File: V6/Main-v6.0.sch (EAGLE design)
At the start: 102 parts, among them J11 AVR_SPI_PROG_3X2NS, M01 JUMPER-SMT_2_NC_PASTE_SILK, M02 JUMPER-SMT_2_NC_PASTE_SILK, M11 JUMPER-SMT_2_NC_PASTE_SILK, M12 JUMPER-SMT_2_NC_PASTE_SILK, Q1 MOSFET-NCHANNEL2N7002PW, Q2 MOSFET-NCHANNEL2N7002PW, U1 ULN2803ADWG4, U10 FSMSMTR, U2 ULN2803ADWG4, U3 UA7805CKTTR, U4 DRV8834RGERTSSOP, U5 DRV8834RGERTSSOP, U7 ATMEGA328P_TQFP, U8 SSA12, U9 FSMSMTR, X1 FH12-16S-1SH, Y1 16MHZ

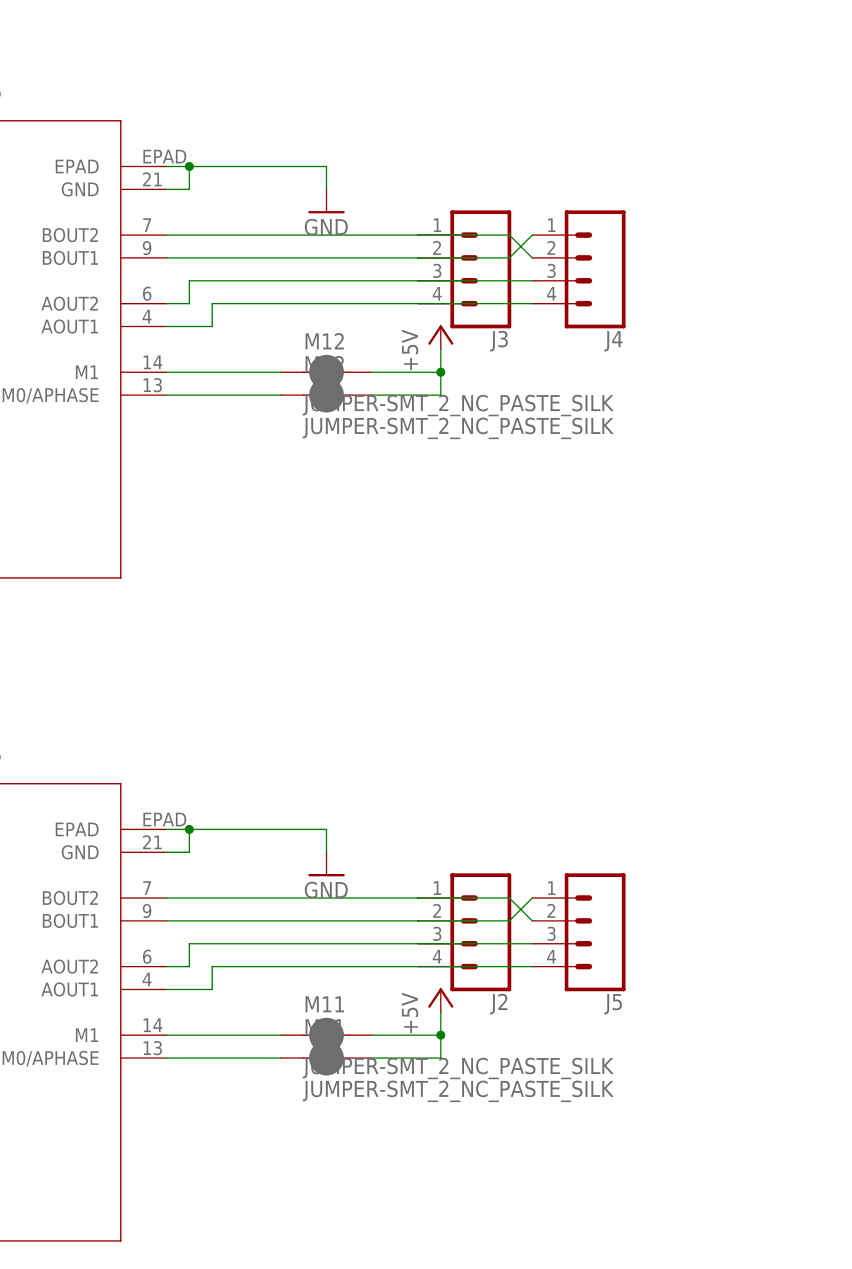
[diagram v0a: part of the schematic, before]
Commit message: V6.0 Updated
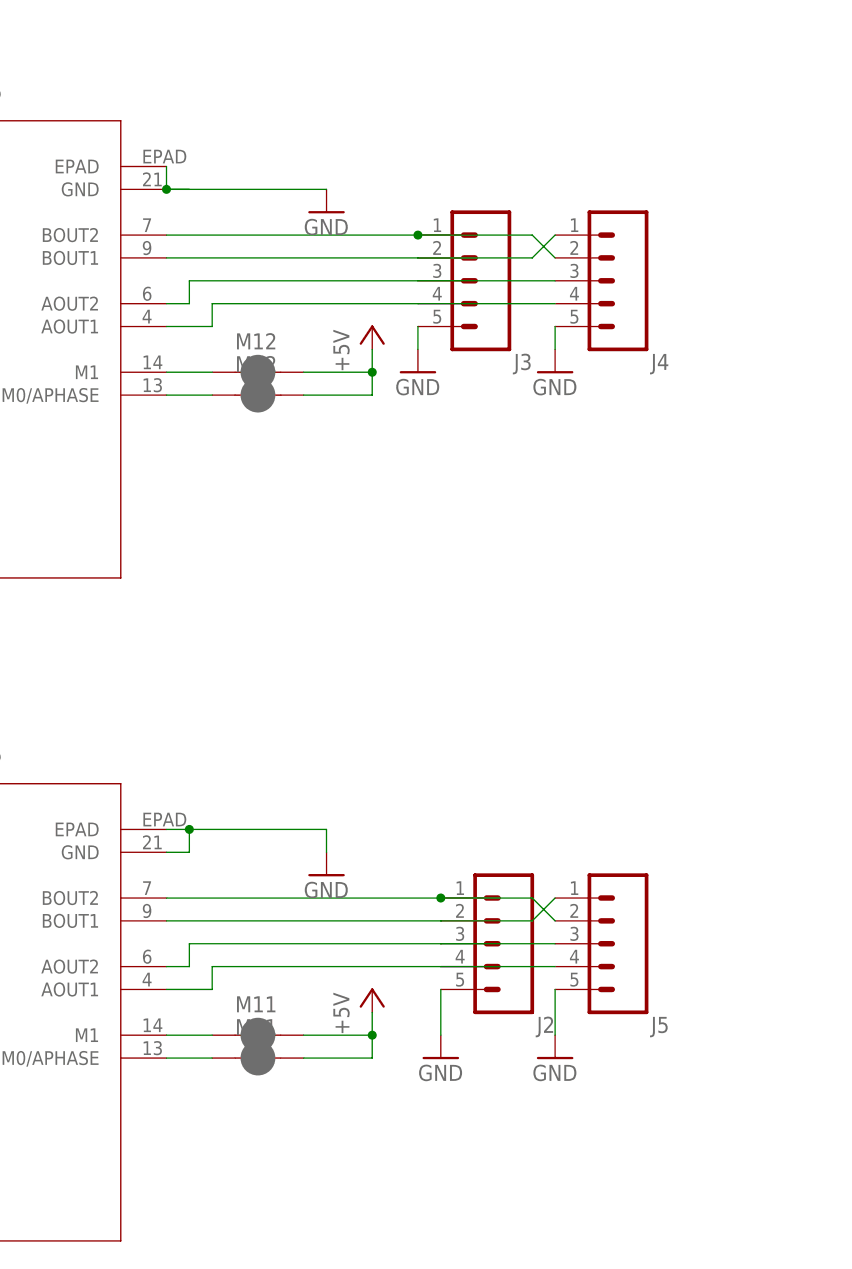
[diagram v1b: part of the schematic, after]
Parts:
- J2, J3, J4, J5: device SparkFun-Connectors:CONN_04 -> SparkFun-Connectors:CONN_05
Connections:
- removed net GND: C1.2, C10.1, C12.1, C13.2, C14.2, C15.2, C16.2, C17.-, C18.2, C19.2, C2.2, C21.2, C22.2, C23.2, C24.-, C3.2, C4.2, C5.2, C6.-, C7.-, J1.1, J10.1, J11.6, J6.1, R10.2, R11.1, R12.1, R14.1, R15.2, R16.2, R17.2, R2.2, R20.1, R21.1, R25.1, R3.2, R34.1, R4.2, R5.2, R6.2, R7.1, S3.O, TM1.A, TM2.A, U$1.INHIBIT, U$1.VSS, U$3.GND, U1.GND, U10.1, U2.GND, U3.COMMON, U3.EPAD, U4.EPAD, U4.GND, U5.EPAD, U5.GND, U6.GND, U7.AGND, U7.GND@3, U7.GND@5, U9.1, VR1.GND, Y1.2
- new net GND_ABC: C1.2, C10.1, C12.1, C13.2, C14.2, C15.2, C16.2, C17.-, C18.2, C19.2, C2.2, C21.2, C22.2, C23.2, C24.-, C3.2, C4.2, C5.2, C6.-, C7.-, J1.1, J10.1, J11.6, J2.5, J3.5, J4.5, J5.5, J6.1, R10.2, R11.1, R12.1, R14.1, R15.2, R16.2, R17.2, R2.2, R20.1, R21.1, R25.1, R3.2, R34.1, R4.2, R5.2, R6.2, R7.1, S3.O, TM1.A, TM2.A, U$1.INHIBIT, U$1.VSS, U$3.GND, U1.GND, U10.1, U2.GND, U3.COMMON, U3.EPAD, U4.EPAD, U4.GND, U5.EPAD, U5.GND, U6.GND, U7.AGND, U7.GND@3, U7.GND@5, U9.1, VR1.GND, Y1.2
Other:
- moved on the sheet: M01, M02, M11, M12

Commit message: V6.0 Updated
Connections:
- net GND_ABC renamed GND
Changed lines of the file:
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@@
 </busses>
 <nets>
-<net name="GND_ABC" class="0">
+<net name="GND" class="0">
 <segment>
 <pinref part="GND1" gate="1" pin="GND"/>
